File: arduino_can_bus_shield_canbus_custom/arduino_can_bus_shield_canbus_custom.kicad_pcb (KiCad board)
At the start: 2 copper layers, 56.4 x 53.3 mm, 47 parts, among them J1 USB_A, J2 jumper, J3 molex_3.0, J4 molex_3.0, J5 UART2, J6 i2C, P1 Power, P2 Analog, P3 Digital, P4 Digital, SW1 User, U1 MCP2515-xST, U2 MAX3421E, U3 74LVC1G125, U4 74LVC1G125, U5 74LVC1G125, U6 74LVC1G125, U7 74LVC1G125, U8 74LVC1G125, U9 MCP2551-I-SN, Y1 Crystal_Small, Y2 16MHz

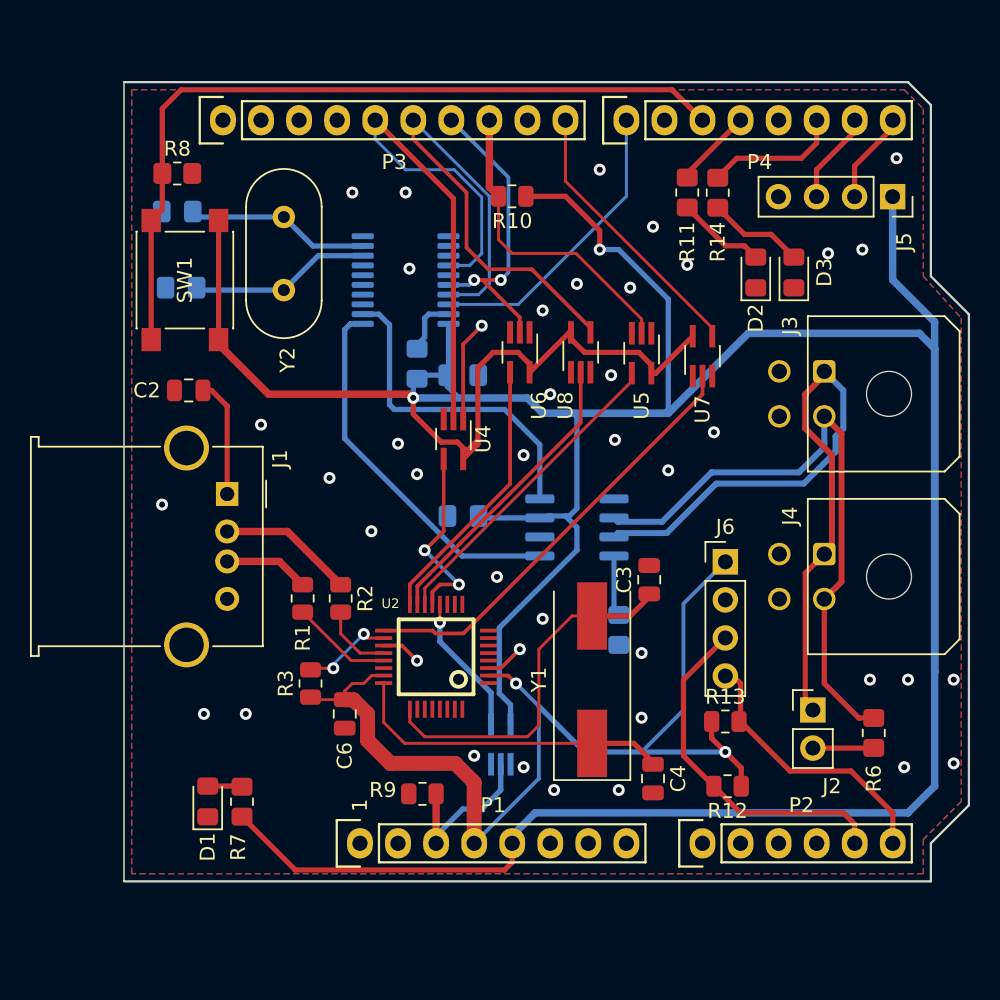
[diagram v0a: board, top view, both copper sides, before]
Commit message: regular update
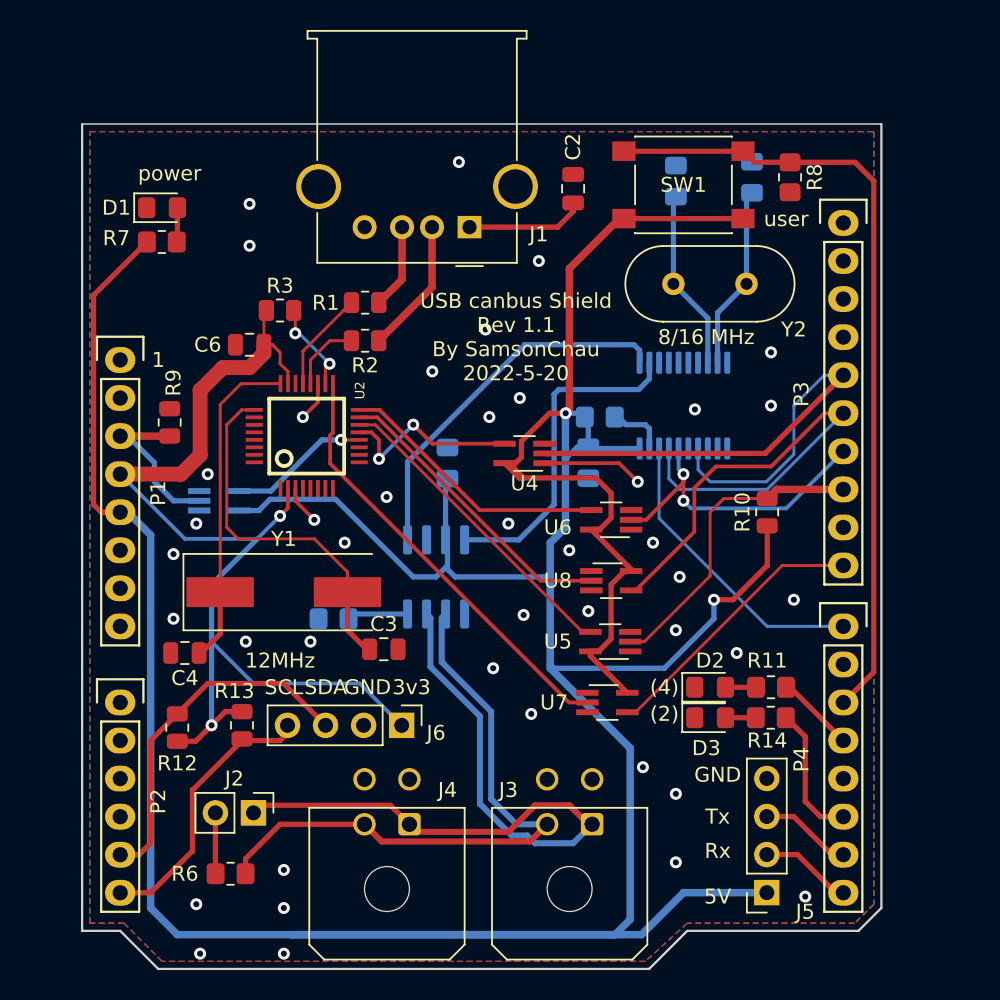
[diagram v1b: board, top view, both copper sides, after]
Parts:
- Y1: value Crystal_Small -> 12MHz
- moved J5 47.2 mm to (128.8, 164.3), turned to 180 degrees
- moved R6 43.9 mm to (93.0, 163.1), turned to 0 degrees
- moved P3 42.0 mm to (133.9, 119.6), turned to -90 degrees
- moved R8 40.9 mm to (130.3, 116.6), turned to -90 degrees
- moved P2 40.0 mm to (85.6, 151.6), turned to -90 degrees
- moved D1 39.7 mm to (88.4, 118.6), turned to 0 degrees
- moved C5 38.4 mm to (127.8, 116.6), turned to 90 degrees
- moved J2 38.0 mm to (94.5, 159.0), turned to -90 degrees
- moved R7 37.7 mm to (88.4, 120.9), turned to 0 degrees
- moved R12 36.9 mm to (89.4, 153.3), turned to 90 degrees
- moved P4 36.8 mm to (133.9, 146.6), turned to -90 degrees
- moved P1 36.0 mm to (85.6, 128.8), turned to -90 degrees
- moved R14 35.2 mm to (129.0, 152.7), turned to 180 degrees
- moved J3 34.0 mm to (117.1, 159.8), turned to 180 degrees
- moved SW1 33.9 mm to (123.2, 117.1), turned to 0 degrees
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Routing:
- net Net-(D3-Pad2): track 6.44 -> 2.02 mm
- net Net-(D2-Pad2): track 5.94 -> 2.04 mm
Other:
- board size 56.4 x 53.3 mm -> 53.3 x 56.4 mm
- board text added: "(2)"
- board text added: "(4)"
- board text added: "12MHz"
- board text added: "3v3"
- board text added: "5V"
- board text added: "8/16 MHz"
- board text added: "GND"
- board text added: "Rx"
- board text added: "SCL"
- board text added: "SDA"
- board text added: "Tx"
- board text added: "USB canbus Shield Rev 1.1 By SamsonChau 2022-5-20"
- board text added: "power"
- board text added: "user"
